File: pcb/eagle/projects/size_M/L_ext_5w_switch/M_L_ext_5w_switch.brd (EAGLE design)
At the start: 10 parts

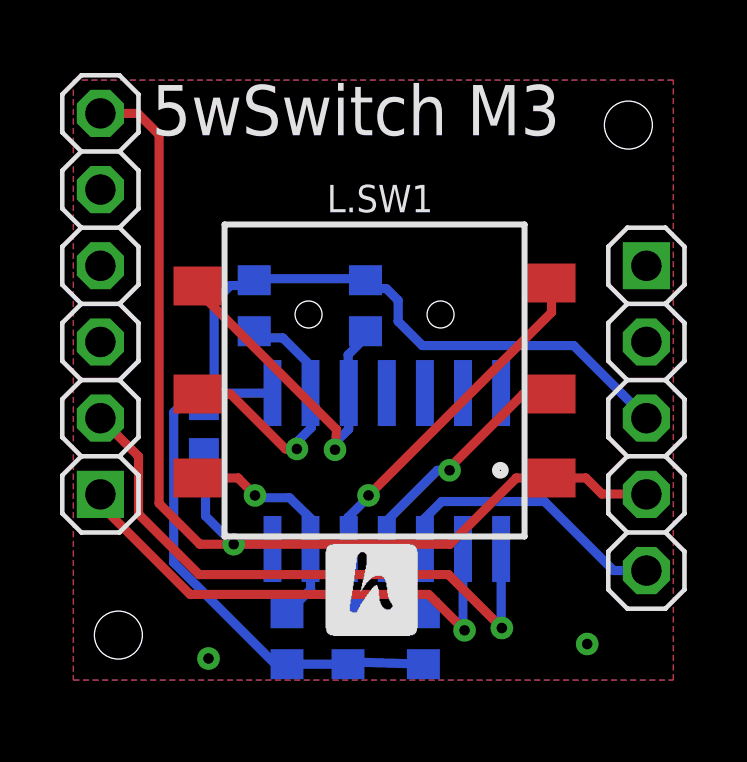
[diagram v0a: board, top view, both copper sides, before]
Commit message: PCB M.3
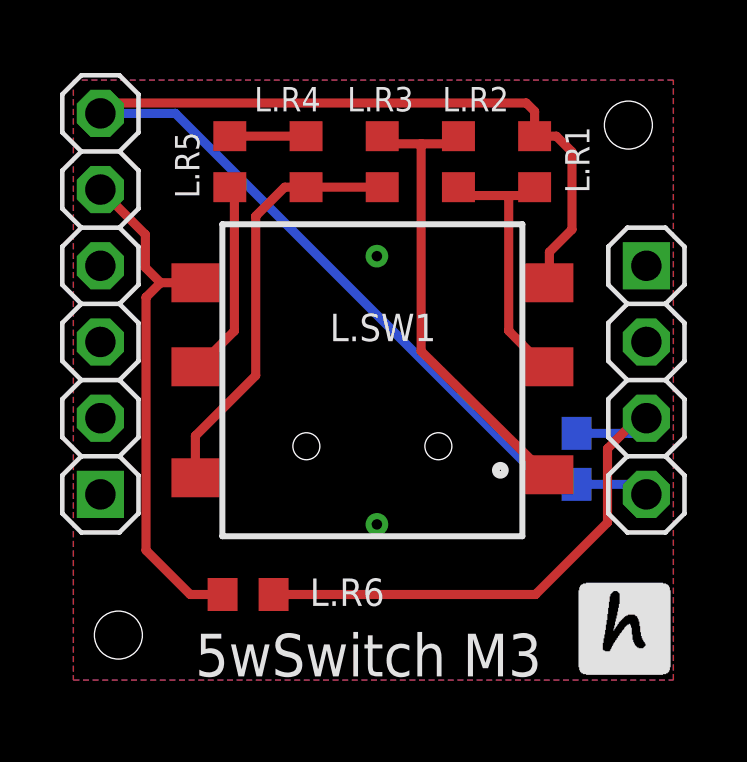
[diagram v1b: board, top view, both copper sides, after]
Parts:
- removed L.U1: AT414, atmel:SO14
- added L.R6: 2k2, rcl:R0603
- G.J2: device pinhead2:1X05 -> pinhead2:1X04
- L.R1, L.R2: value (none) -> 1k
- L.R3, L.R4, L.R5: value (none) -> 2k2
- moved L.R1 16.3 mm to (15.9, 17.8), flipped to the top
- moved L.R2 16.3 mm to (13.3, 17.8), flipped to the top, turned to 270 degrees
- moved L.R3 16.2 mm to (10.8, 17.8), flipped to the top, turned to 90 degrees
- moved L.C1 12.5 mm to (17.3, 7.87)
- moved L.R5 6.59 mm to (5.71, 17.8), flipped to the top, turned to 270 degrees
- moved L.R4 5.10 mm to (8.26, 17.8), flipped to the top, turned to 270 degrees
- moved G.J2 1.27 mm to (19.6, 10.5)
- moved L.SW1 0.52 mm to (10.6, 10.7), turned to 0 degrees
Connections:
- removed net N$2: G.J1.2, L.U1.8
- removed net N$3: G.J2.5, L.U1.10
- removed net N$9: L.R1.2, L.SW1.2, L.U1.11
- new net N$4: L.R1.1, L.R2.2, L.SW1.5
- net GND: now also L.R1.2, L.SW1.4; no longer L.SW1.1, L.U1.14
- net N$1: now also L.R4.1, L.R5.1; no longer G.J1.1, L.U1.9
- net N$5: now also L.R2.1, L.R3.2; no longer L.R5.1, L.U1.3
- net N$6: now also L.R3.1, L.R4.2, L.SW1.3; no longer L.R4.1, L.SW1.5, L.U1.2
- net N$7: now also G.J1.5, L.R6.1, L.SW1.1; no longer L.R3.1, L.SW1.4, L.U1.13
- net N$8: now also L.R5.2, L.SW1.2; no longer L.R2.2, L.SW1.3, L.U1.12
- net VCC: now also L.R6.2; no longer L.R1.1, L.R2.1, L.R3.2, L.R4.2, L.R5.2, L.U1.1
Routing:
- net VCC: track 39.7 -> 18.8 mm
- net N$2: track 20.0 -> 0.00 mm, vias 1 -> 0
- net N$1: track 16.9 -> 2.62 mm, vias 1 -> 0
- net N$9: track 10.9 -> 0.00 mm, vias 1 -> 0
- net N$3: track 9.59 -> 0.00 mm
- net N$7: track 7.82 -> 17.4 mm, vias 1 -> 0
- net N$4: track 0.00 -> 9.19 mm
- net GND: track 37.2 -> 45.2 mm, vias 3 -> 2
- net N$8: track 14.2 -> 6.62 mm, vias 1 -> 0
- net N$6: track 9.41 -> 14.2 mm, vias 1 -> 0
- net N$5: track 11.8 -> 15.7 mm, vias 1 -> 0
